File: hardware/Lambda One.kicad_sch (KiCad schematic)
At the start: 26 parts, among them IC1 01, J1 Conn_01x02, SW1 SW_Push, U1 W65C816SxP, U3 ATF22LV10C, U8 74HC00, Y1 TFT680

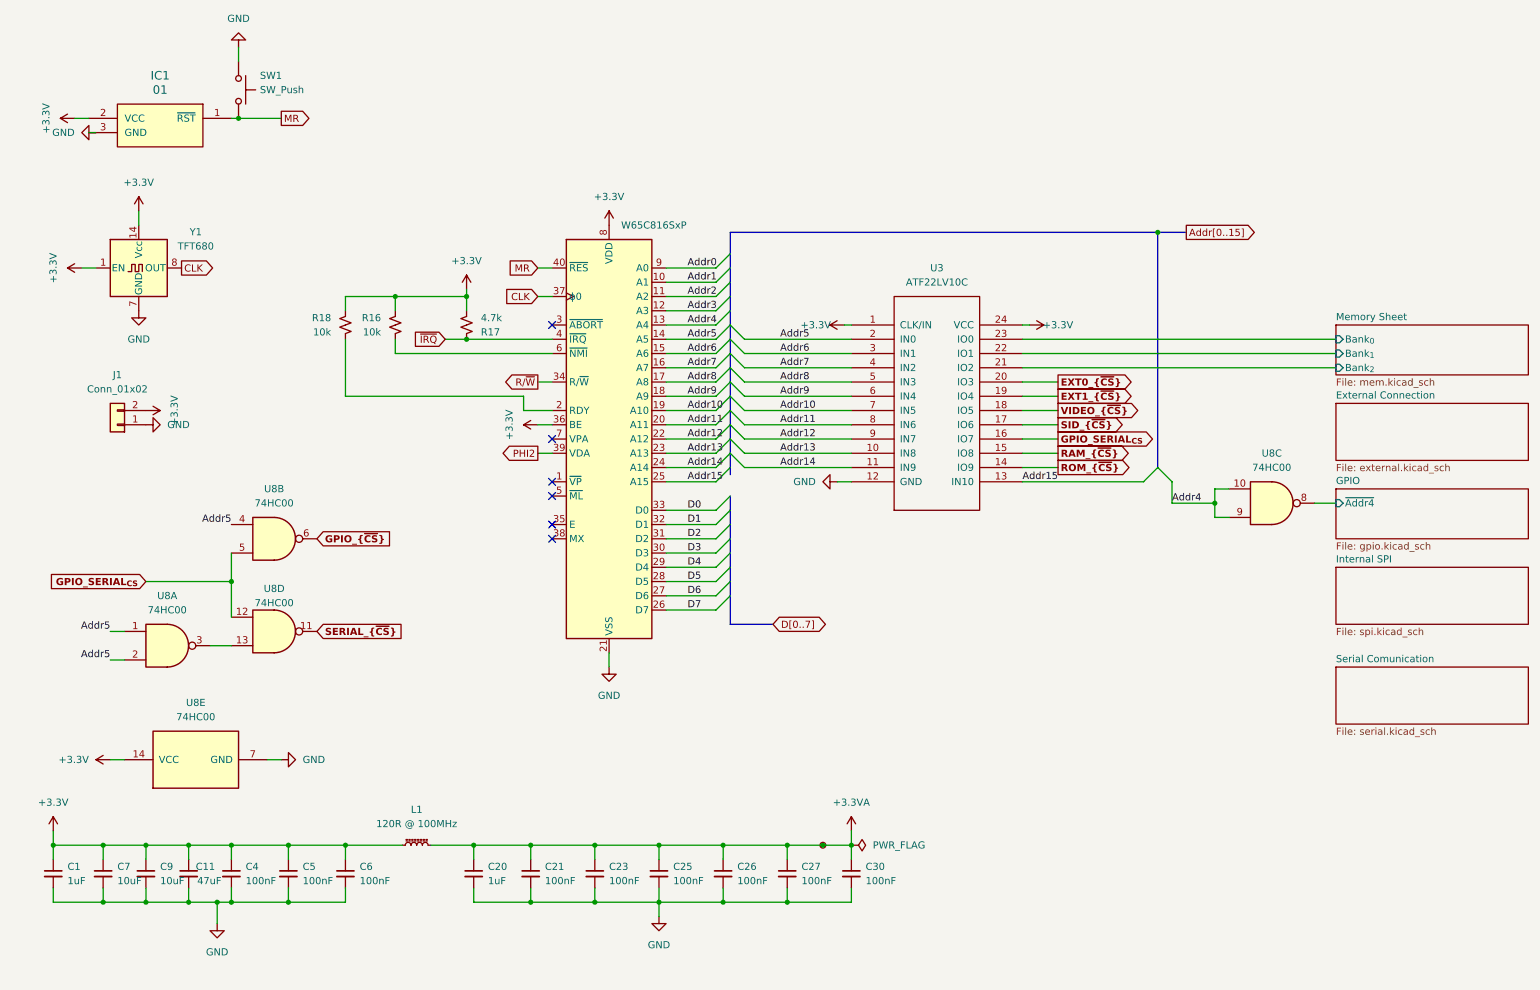
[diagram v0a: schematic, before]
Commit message: Fixes and addres fix adding VDA AND VPA
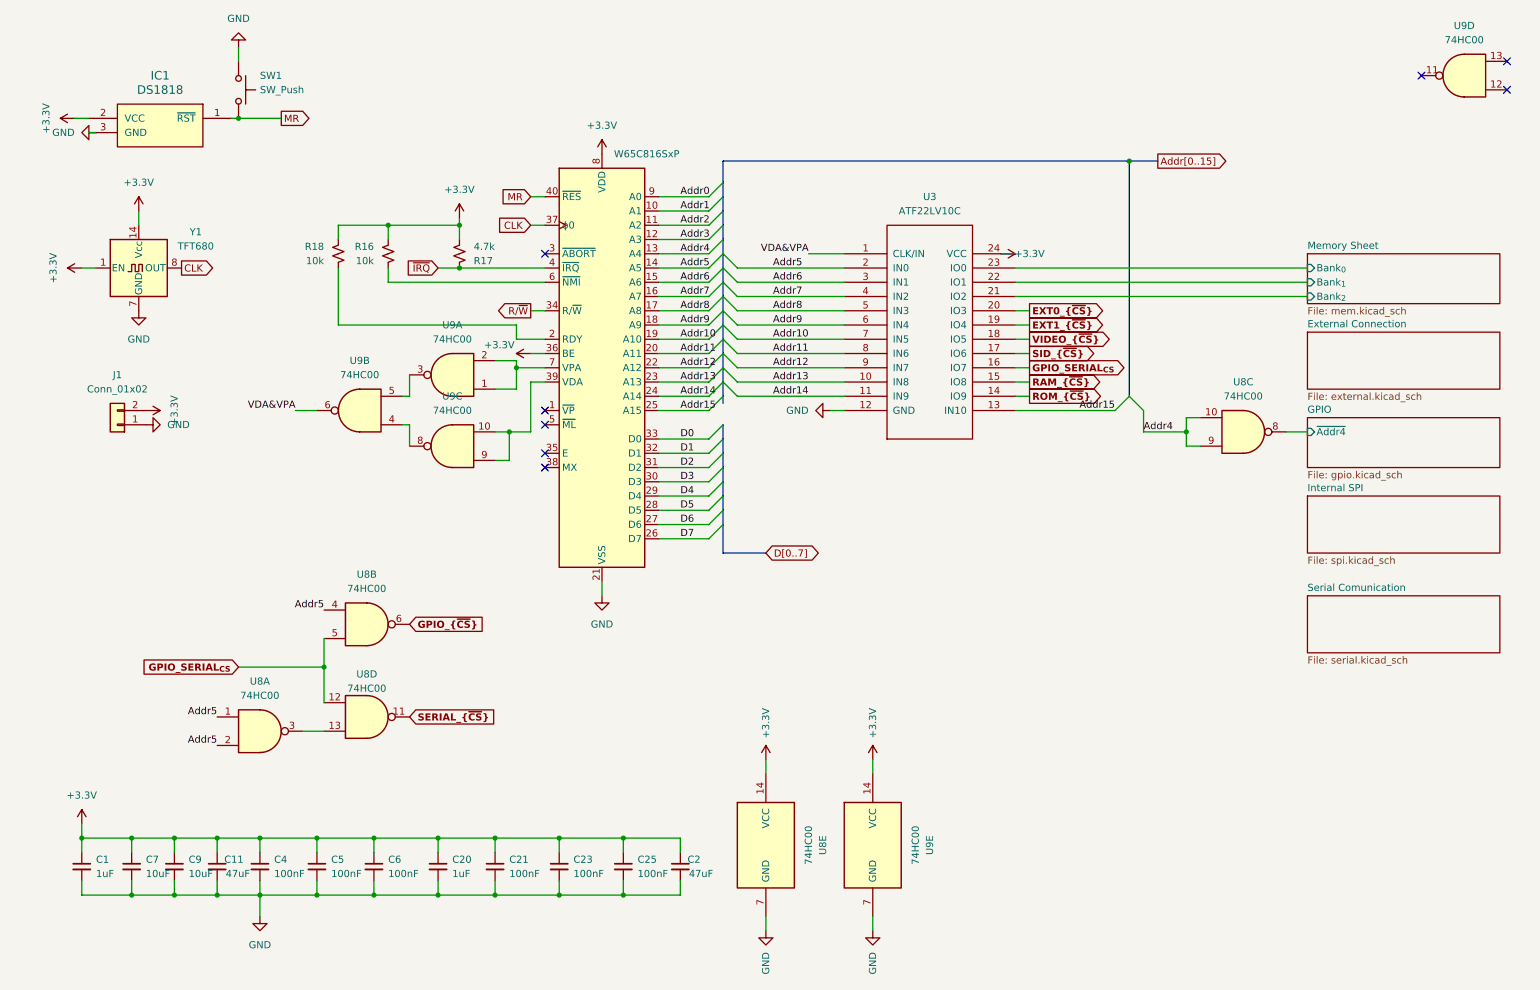
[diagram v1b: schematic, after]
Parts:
- removed C26, C27, C30: 100nF, Capacitor_SMD:C_0603_1608Metric, symbol Device:C_Small
- removed L1: 120R @ 100MHz, Inductor_SMD:L_0603_1608Metric, symbol Device:L_Ferrite_Small
- removed TP13: TestPoint_Small, TestPoint:TestPoint_Pad_D1.5mm, symbol Connector:TestPoint_Small
- added C2: 47uF, Capacitor_SMD:C_0603_1608Metric, symbol Device:C_Small
- added U9: 74HC00, symbol 74xx:74HC00
- IC1: value 01 -> DS1818
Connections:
- net +3.3VA is gone; now on net +3.3V: C20.1, C21.1, C23.1, C25.1
- net +3.3V: now also C2.1, U9.14 (VCC); no longer U3.1 (CLK/IN)
- net GND: now also C2.2, U9.7 (GND)
- net at U1.7 (VPA): now also U9.1, U9.2
- net PHI2: no longer names the net of U1.39 (VDA)
- net PHI2: now also U9.10, U9.9
- new net: U9.4, U9.8
- new net: U9.3, U9.5
- new net VDA&VPA: U3.1 (CLK/IN), U9.6
- no-connect marks 6 -> 8
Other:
- moved on the sheet: C1, C11, C20, C21, C23, C25, C4, C5, C6, C7, C9, R16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
